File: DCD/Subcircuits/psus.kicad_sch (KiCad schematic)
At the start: 18 parts, among them U3 LP2985-18DBVR, U5 LP2985-33DBVR, U6 LP2985-50DBVR

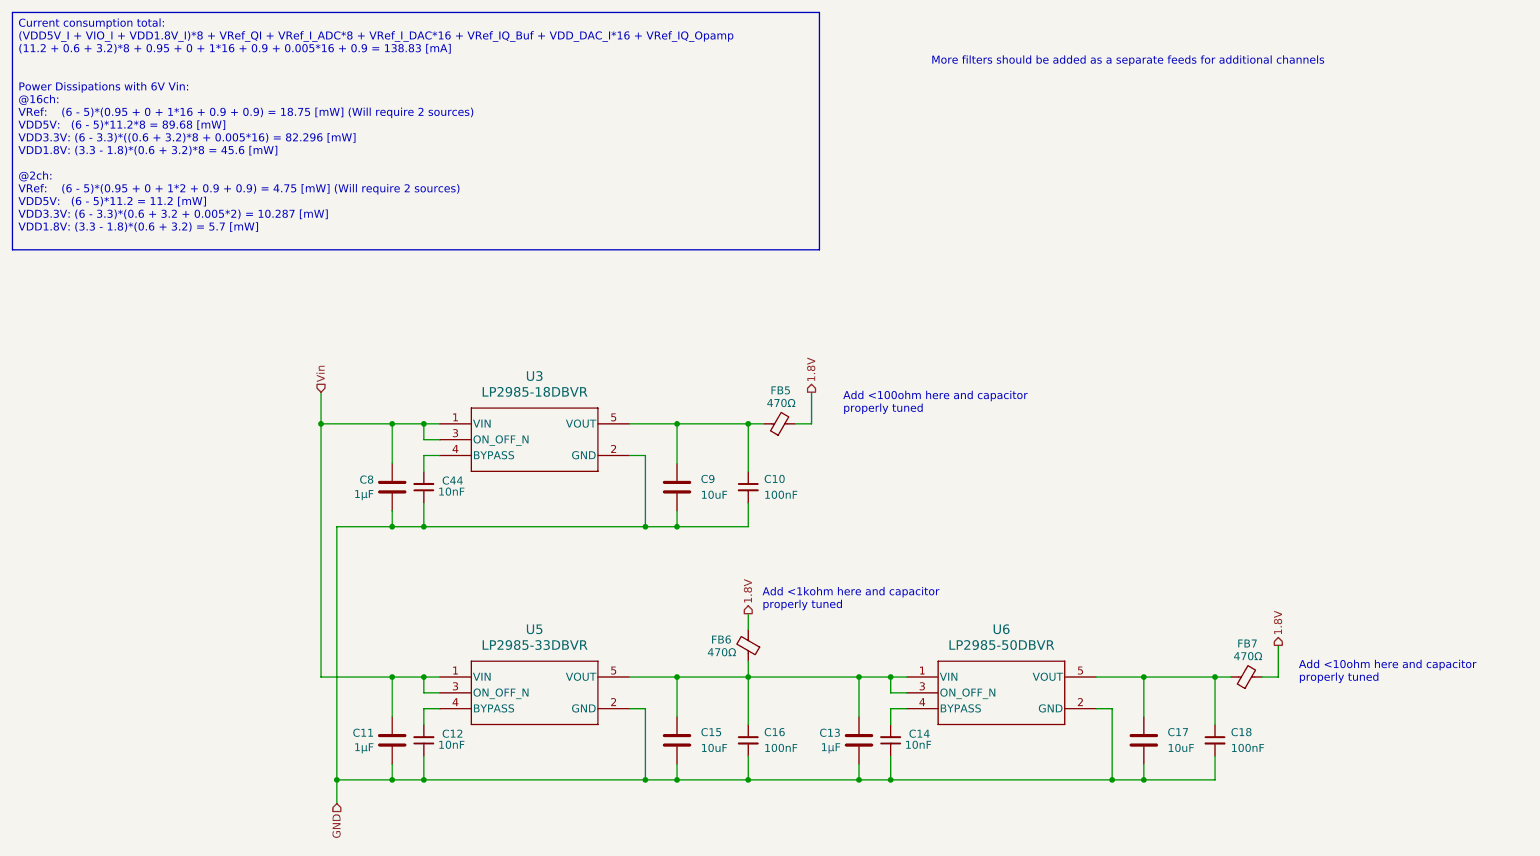
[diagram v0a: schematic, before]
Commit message: Finished the schematics. Fixed the comments that we recieved
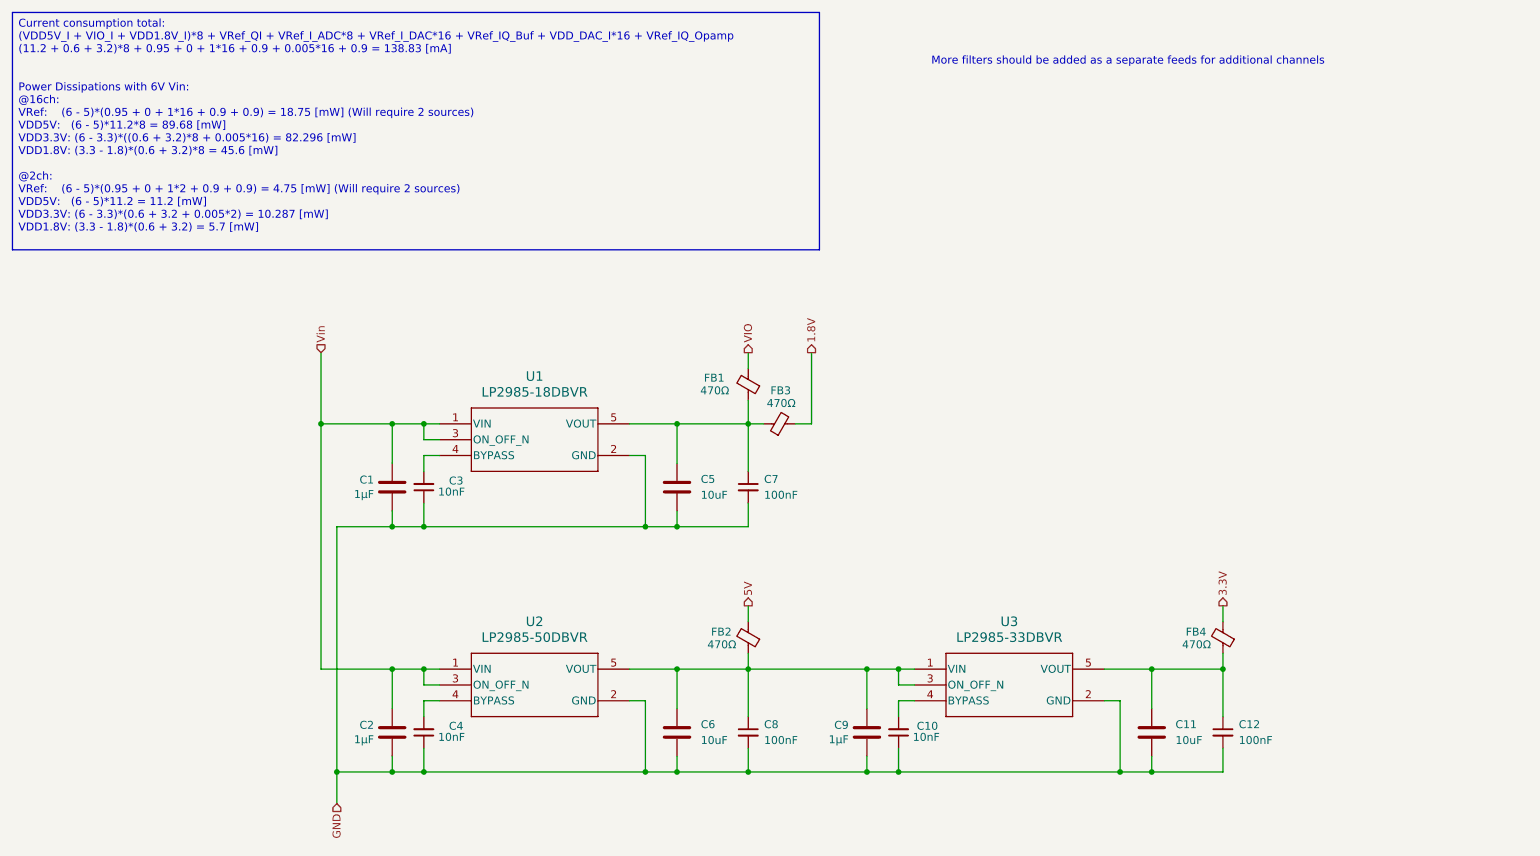
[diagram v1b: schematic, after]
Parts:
- added FB1: 470Ω, Inductor_SMD:L_0603_1608Metric, symbol Device:FerriteBead_Small
- renumbered C8 to C1, C12 to C10, C15 to C11, C16 to C12, C13 to C2, C44 to C3, C14 to C4, C9 to C5, C17 to C6, C10 to C7, C18 to C8, C11 to C9, FB7 to FB2, FB5 to FB3, FB6 to FB4, U3 to U1, U6 to U2, U5 to U3
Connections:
- net 1.8V: no longer FB2.2, FB4.2
- net Vin: now also C2.1, U2.1 (VIN), U2.3 (ON_OFF_N); no longer C9.1, U3.1 (VIN), U3.3 (ON_OFF_N)
- net at C11.1, C12.1, FB4.1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: no longer C2.1, U2.1 (VIN), U2.3 (ON_OFF_N)
- net at C5.1, C7.1, FB3.1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: now also FB1.1
- net at C6.1, C8.1, FB2.1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: now also C9.1, U3.1 (VIN), U3.3 (ON_OFF_N)
- new net 3.3V: FB4.2
- new net 5V: FB2.2
- new net VIO: FB1.2
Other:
- note removed: "Add <100ohm here and capacitor properly tuned"
- note removed: "Add <10ohm here and capacitor properly tuned"
- note removed: "Add <1kohm here and capacitor properly tuned"
- moved on the sheet: C10, C11, C12, C2, C4, C6, C8, C9, FB2, FB4, U2, U3
